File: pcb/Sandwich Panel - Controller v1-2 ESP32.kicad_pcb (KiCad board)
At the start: 2 copper layers, 140 x 50 mm, 28 parts, among them J1 Conn_01x02_Male, J2 Conn_01x02_Male, J4 Conn_01x04, J5 USB_C_Receptacle_USB2.0, U1 ESP32-S3-MINI-1-N8, U2 SPX3819M5-L-3-3

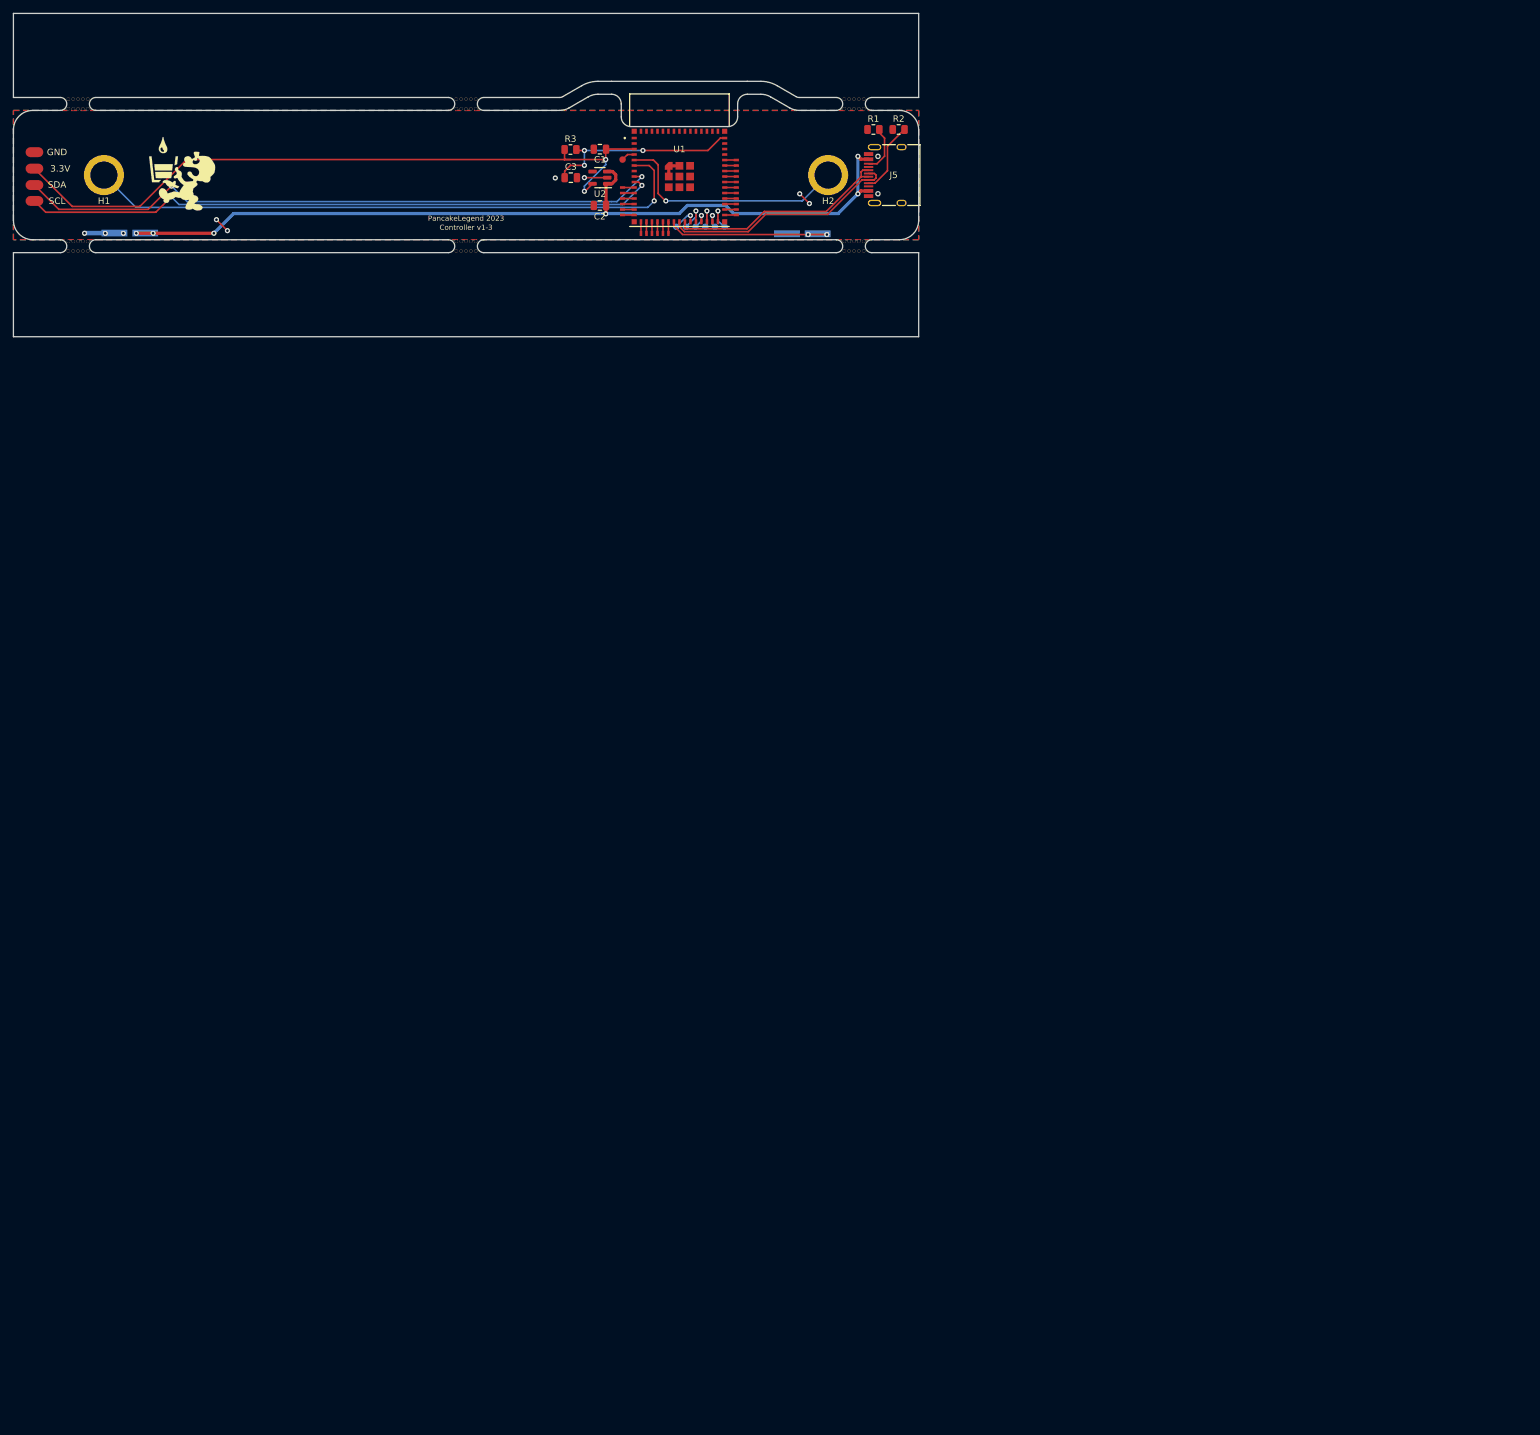
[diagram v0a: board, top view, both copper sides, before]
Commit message: Old zones don't seem to be removable, will edit the text file next, wish me luck
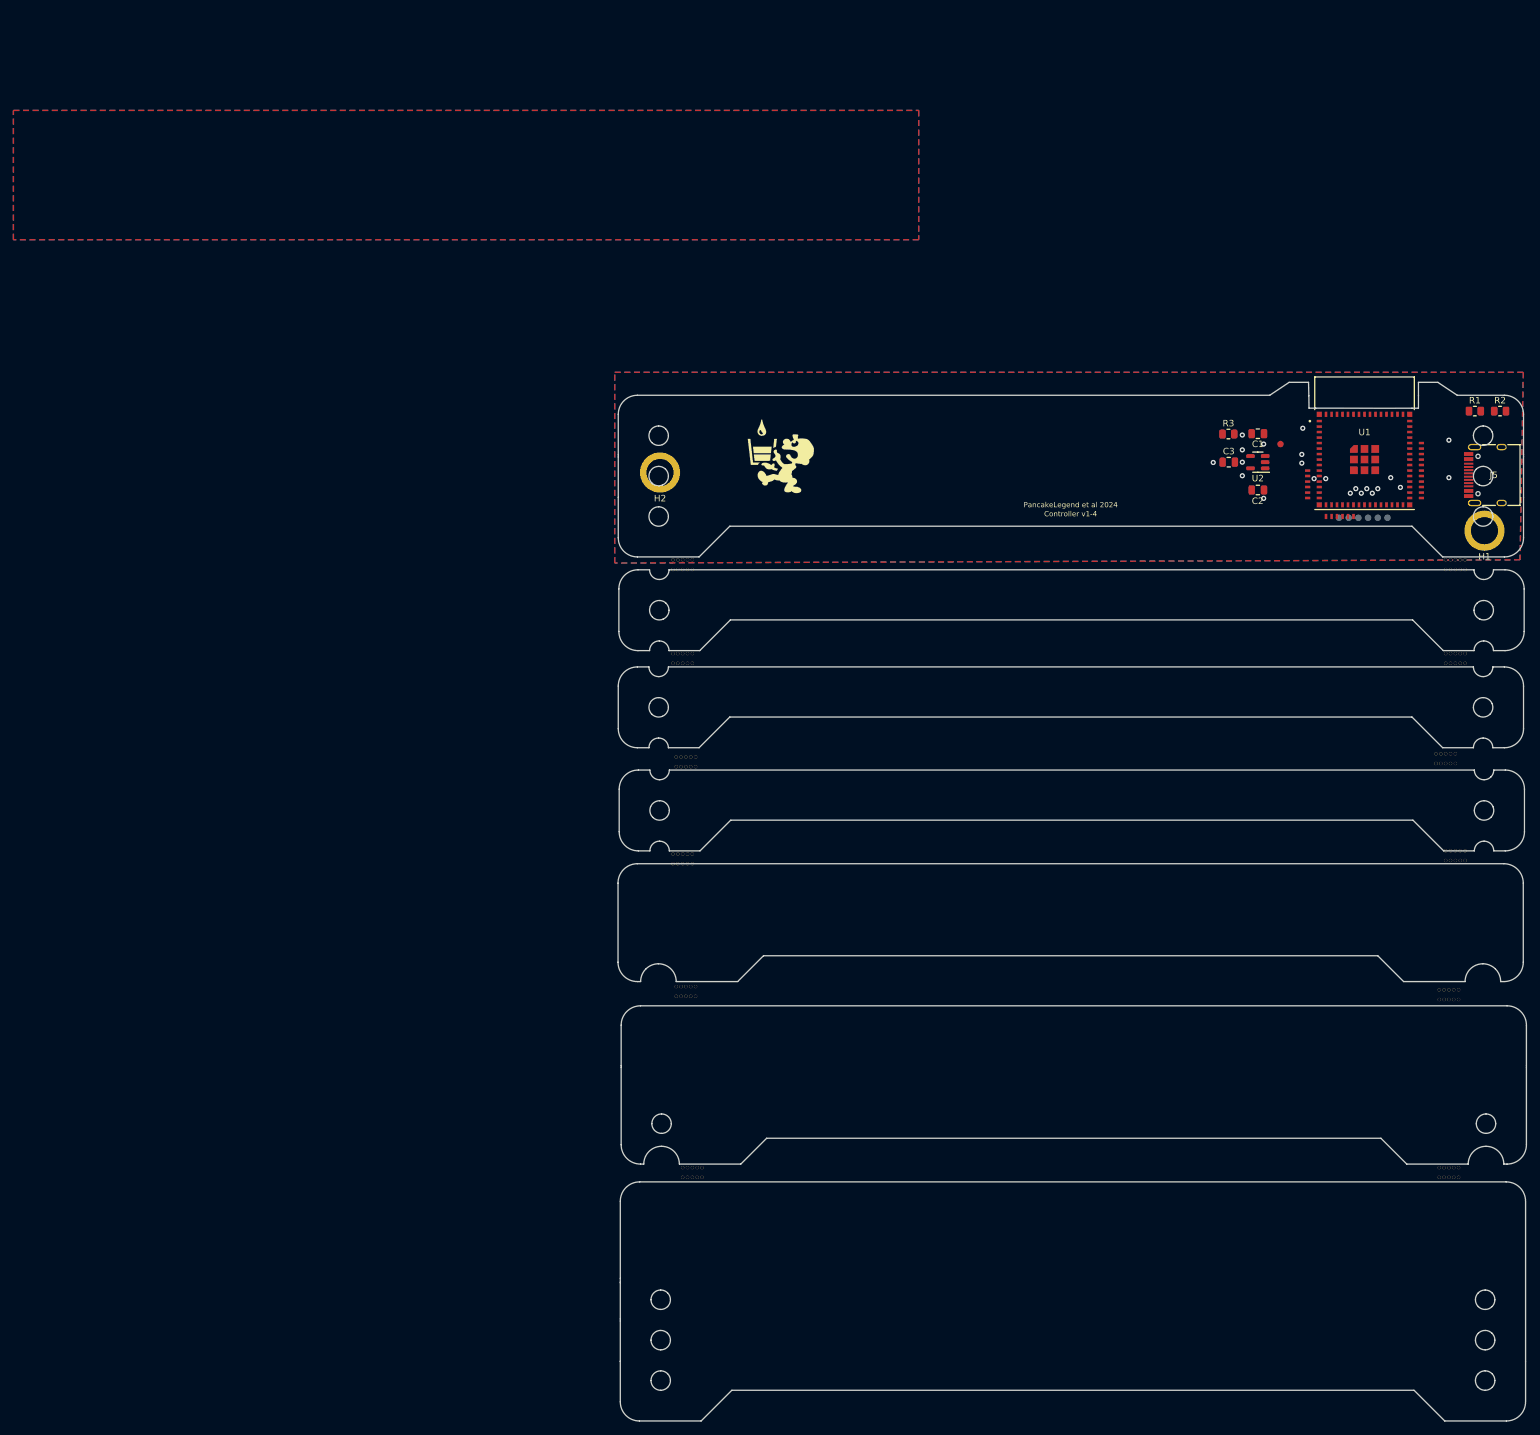
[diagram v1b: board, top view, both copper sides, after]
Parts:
- removed H4, H5, H6, H7, H8: Mousebites, Pancake:Mousebites_03
- removed J1, J2: Conn_01x02_Male, Pancake:Panel_Connector 02
- removed J4: Conn_01x04, Pancake:I2C Breakout Pads
- added H3: Mousebites, Pancake:Mousebites_03, F.Cu at (33.5, 64.8)
- added H3: Mousebites, Pancake:Mousebites_03, F.Cu at (153.0, 95.2)
- added H3: Mousebites, Pancake:Mousebites_03, F.Cu at (35.0, 144.2)
- added H3: Mousebites, Pancake:Mousebites_03, F.Cu at (153.0, 50.2)
- added H3: Mousebites, Pancake:Mousebites_03, F.Cu at (152.0, 144.2)
- added H3: Mousebites, Pancake:Mousebites_03, F.Cu at (152.0, 116.8)
- added H3: Mousebites, Pancake:Mousebites_03, F.Cu at (34.0, 116.2)
- added H3: Mousebites, Pancake:Mousebites_03, F.Cu at (33.5, 95.8)
- added H3: Mousebites, Pancake:Mousebites_03, F.Cu at (153.0, 64.8)
- added H3: Mousebites, Pancake:Mousebites_03, F.Cu at (151.5, 80.2)
- added H3: Mousebites, Pancake:Mousebites_03, F.Cu at (34.0, 80.8)
- moved H1 220.5 mm to (157.5, 45.0)
- moved H3 117.6 mm to (33.5, 50.2)
- moved U1 114.6 mm to (138.9, 34.0)
- moved TP2 111.9 mm to (135.0, 43.0)
- moved TP3 111.9 mm to (136.5, 43.0)
- moved TP4 111.9 mm to (138.0, 43.0)
- moved TP5 111.9 mm to (139.5, 43.0)
- moved TP6 111.9 mm to (141.0, 43.0)
- moved TP7 111.9 mm to (142.5, 43.0)
- moved C1 110.9 mm to (122.5, 30.0)
- moved C2 110.9 mm to (122.5, 38.7)
- moved C3 110.9 mm to (118.0, 34.4)
- moved R3 110.9 mm to (117.9, 30.1)
- moved TP1 110.9 mm to (126.0, 31.6)
- moved U2 110.9 mm to (122.5, 34.4)
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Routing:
- net +5V: track 133.6 -> 0.00 mm, vias 6 -> 2
- net 3.3V: track 110.3 -> 0.00 mm
- net SDA: track 100.8 -> 0.00 mm, vias 2 -> 1
- net SCL: track 98.8 -> 0.00 mm, vias 2 -> 1
- net Net-(H1-Pad1): track 95.7 -> 0.00 mm
- net Net-(H2-Pad1): track 36.8 -> 0.00 mm
- net D-: track 36.6 -> 0.00 mm
- net D+: track 34.7 -> 0.00 mm
- net Net-(C3-Pad1): track 30.2 -> 0.00 mm
- net DOUT: track 24.8 -> 0.00 mm, vias 2 -> 0
- net GND: track 16.0 -> 0.00 mm, vias 9 -> 4
- net Net-(J5-PadA5): track 11.1 -> 0.00 mm
- net Net-(J5-PadB5): track 7.37 -> 0.00 mm
- net Net-(U1-Pad26): track 4.77 -> 0.00 mm
- net Net-(U1-Pad30): track 4.62 -> 0.00 mm
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- added copper zone on F.Cu, net +5V
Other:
- board size 140 x 50 mm -> 140.5 x 160.6 mm
- board text added: "Controller v1-4"
- board text added: "PancakeLegend et al 2024"
- board text removed: "Controller v1-3"
- board text removed: "JLCJLCJLCJLC"
- board text removed: "PancakeLegend 2023"
